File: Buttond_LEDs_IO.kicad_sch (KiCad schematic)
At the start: 14 parts, among them J13 SFH11-PBPC-D05-ST-BK, SW1 RESET, SW2 BOOT

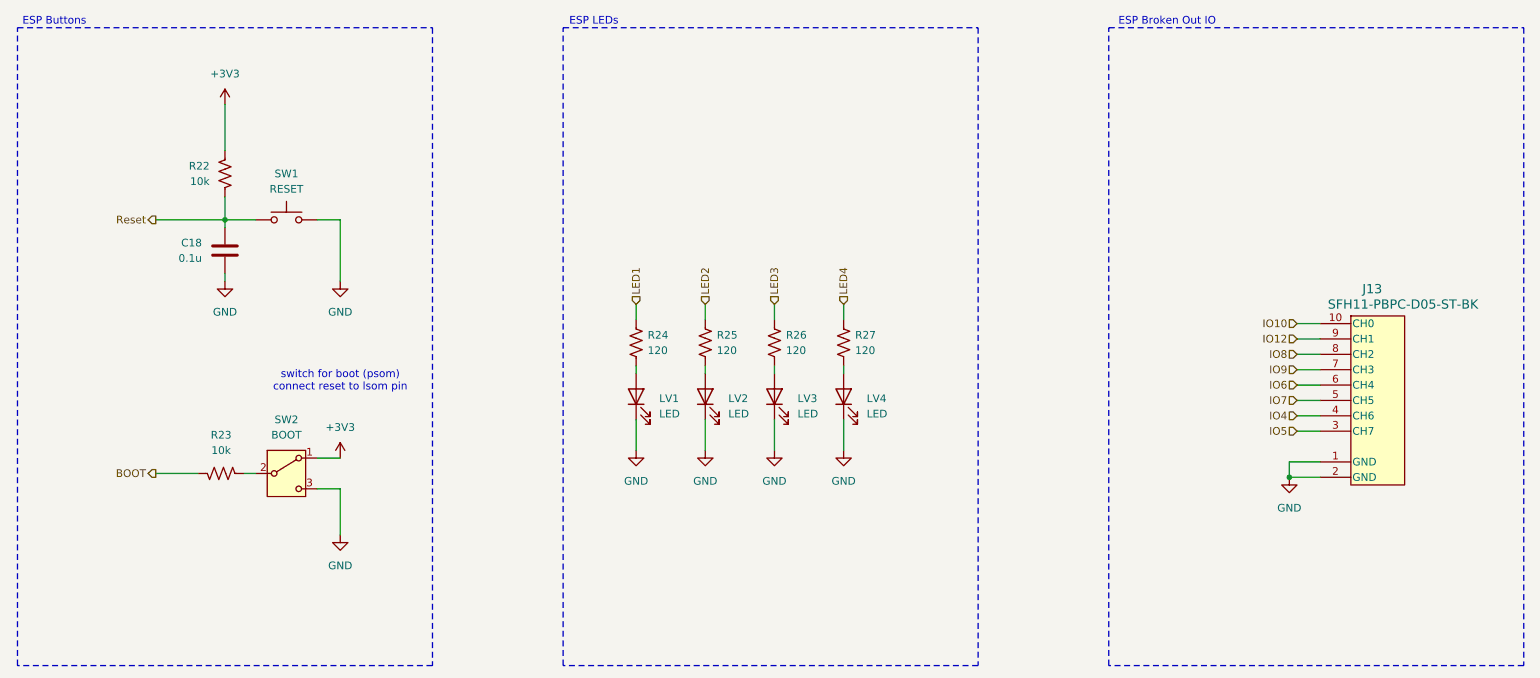
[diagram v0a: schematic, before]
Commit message: start of RevB. BOM for revA
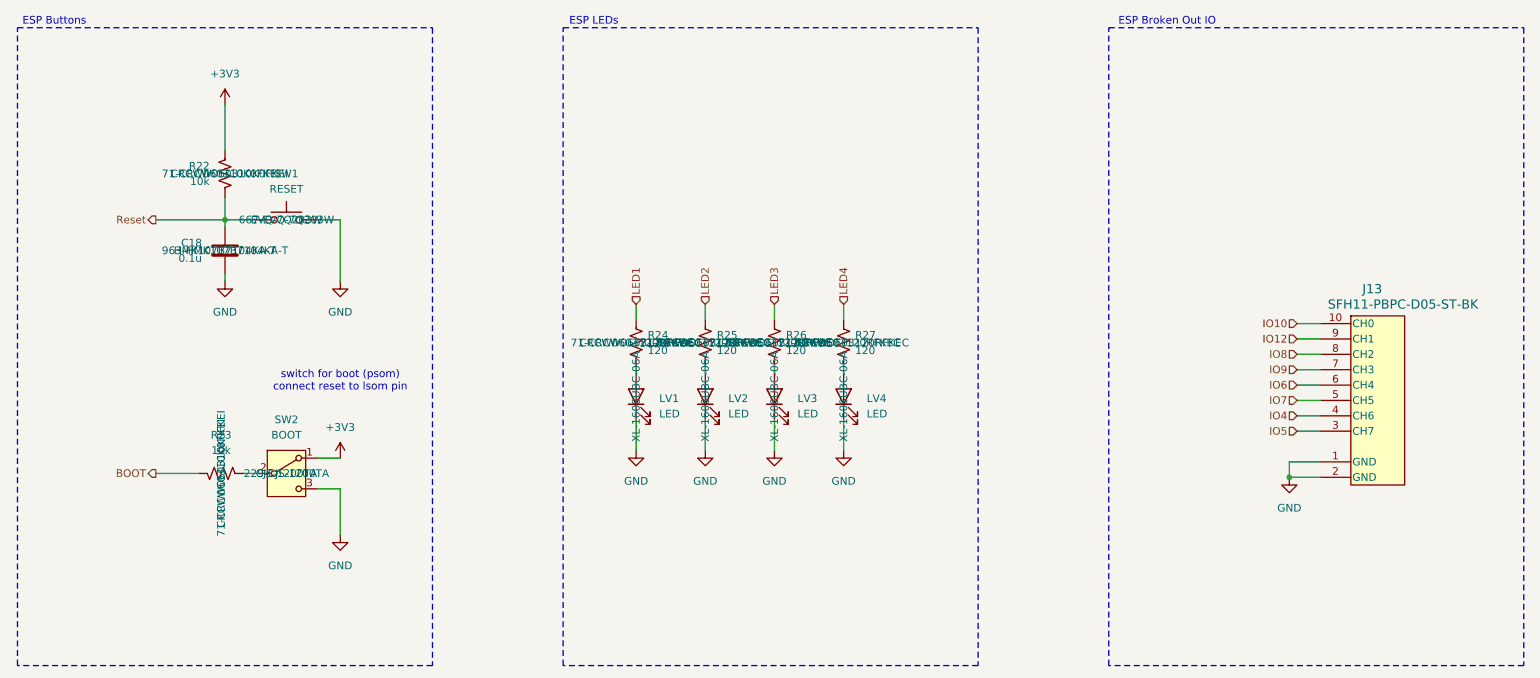
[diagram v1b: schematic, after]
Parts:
- C18: Mouser Part Number (none) -> 963-HMK107B7104KA-T; P/N (none) -> HMK107B7104KA-T
- LV1, LV2, LV3, LV4: P/N (none) -> XL-1608UBC-06A
- R22, R23: Mouser Part Number (none) -> 71-CRCW060310K0FKEI; P/N (none) -> CRCW060310K0FKEI
- R24, R25, R26, R27: Mouser Part Number (none) -> 71-CRCW0603120RFKEC; P/N (none) -> CRCW0603120RFKEC
- SW1: Mouser Part Number (none) -> 667-EVQ-7Q203W; P/N (none) -> EVQ-7Q203W
- SW2: Mouser Part Number (none) -> 229-CJS-1200TA; P/N (none) -> CJS-1200TA
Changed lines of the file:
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@@
+			)
+		)
+		(property "P/N" "CJS-1200TA"
+			(at 71.12 105.41 0)
+			(effects
+				(font
+					(size 1.27 1.27)
+				)
+			)
+		)
+		(property "Mouser Part Number" "229-CJS-1200TA"
+			(at 71.12 105.41 0)
+			(effects
+				(font
+					(size 1.27 1.27)
+				)
 			)
 		)
@@
 			)
 		)
+		(property "P/N" "XL-1608UBC-06A"
+			(at 128.905 92.71 0)
+			(effects
+				(font
+					(size 1.27 1.27)
+				)
+			)
+		)
 		(pin "1"
 		)
@@
 				)
 				(hide yes)
+			)
+		)
+		(property "P/N" "CRCW0603120RFKEC"
+			(at 128.905 83.82 0)
+			(effects
+				(font
+					(size 1.27 1.27)
+				)
+			)
+		)
+		(property "Mouser Part Number" " 71-CRCW0603120RFKEC"
+			(at 128.905 83.82 0)
+			(effects
+				(font
+					(size 1.27 1.27)
+				)
 			)
 		)
@@
 			)
 		)
+		(property "P/N" "HMK107B7104KA-T"
+			(at 60.96 68.58 0)
+			(effects
+				(font
+					(size 1.27 1.27)
+				)
+			)
+		)
+		(property "Mouser Part Number" "963-HMK107B7104KA-T"
+			(at 60.96 68.58 0)
+			(effects
+				(font
+					(size 1.27 1.27)
+				)
+			)
+		)
 		(pin "1"
 		)
@@
 			)
 		)
+		(property "P/N" "CRCW060310K0FKEI"
+			(at 60.96 55.88 0)
+			(effects
+				(font
+					(size 1.27 1.27)
+				)
+			)
+		)
+		(property "Mouser Part Number" "71-CRCW060310K0FKEI"
+			(at 60.96 55.88 0)
+			(effects
+				(font
+					(size 1.27 1.27)
+				)
+			)
+		)
 		(pin "1"
 		)
@@
 			)
 		)
+		(property "P/N" "CRCW0603120RFKEC"
+			(at 140.335 83.82 0)
+			(effects
+				(font
+					(size 1.27 1.27)
+				)
+			)
+		)
+		(property "Mouser Part Number" " 71-CRCW0603120RFKEC"
+			(at 140.335 83.82 0)
+			(effects
+				(font
+					(size 1.27 1.27)
+				)
+			)
+		)
 		(pin "1"
 		)
@@
 				)
 				(hide yes)
+			)
+		)
+		(property "P/N" "XL-1608UBC-06A"
+			(at 140.335 92.71 0)
+			(effects
+				(font
+					(size 1.27 1.27)
+				)
 			)
 		)
@@
 			)
 		)
+		(property "P/N" "CRCW0603120RFKEC"
+			(at 151.765 83.82 0)
+			(effects
+				(font
+					(size 1.27 1.27)
+				)
+			)
+		)
+		(property "Mouser Part Number" " 71-CRCW0603120RFKEC"
+			(at 151.765 83.82 0)
+			(effects
+				(font
+					(size 1.27 1.27)
+				)
+			)
+		)
 		(pin "1"
 		)
@@
 				)
 				(hide yes)
+			)
+		)
+		(property "P/N" "CRCW0603120RFKEC"
+			(at 163.195 83.82 0)
+			(effects
+				(font
+					(size 1.27 1.27)
+				)
+			)
+		)
+		(property "Mouser Part Number" " 71-CRCW0603120RFKEC"
+			(at 163.195 83.82 0)
+			(effects
+				(font
+					(size 1.27 1.27)
+				)
 			)
 		)
@@
 			)
 		)
+		(property "P/N" "EVQ-7Q203W"
+			(at 71.12 63.5 0)
+			(effects
+				(font
+					(size 1.27 1.27)
+				)
+			)
+		)
+		(property "Mouser Part Number" "667-EVQ-7Q203W"
+			(at 71.12 63.5 0)
+			(effects
+				(font
+					(size 1.27 1.27)
+				)
+			)
+		)
 		(pin "2"
 		)
@@
 				)
 				(hide yes)
+			)
+		)
+		(property "P/N" "XL-1608UBC-06A"
+			(at 163.195 92.71 0)
+			(effects
+				(font
+					(size 1.27 1.27)
+				)
 			)
 		)
@@
 			)
 		)
+		(property "P/N" "XL-1608UBC-06A"
+			(at 151.765 92.71 0)
+			(effects
+				(font
+					(size 1.27 1.27)
+				)
+			)
+		)
 		(pin "1"
 		)
@@
 			)
 		)
+		(property "P/N" "CRCW060310K0FKEI"
+			(at 60.325 105.41 0)
+			(effects
+				(font
+					(size 1.27 1.27)
+				)
+			)
+		)
+		(property "Mouser Part Number" "71-CRCW060310K0FKEI"
+			(at 60.325 105.41 0)
+			(effects
+				(font
+					(size 1.27 1.27)
+				)
+			)
+		)
